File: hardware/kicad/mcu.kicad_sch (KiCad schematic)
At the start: 34 parts, among them J3 SWD, J4 UART, J5 Reset_Switch, SW2 PEC11R-4220F-S0024, U6 OLED, U7 STM32F072CBTx, U8 PCT2075GV, Y1 Crystal_8MHz

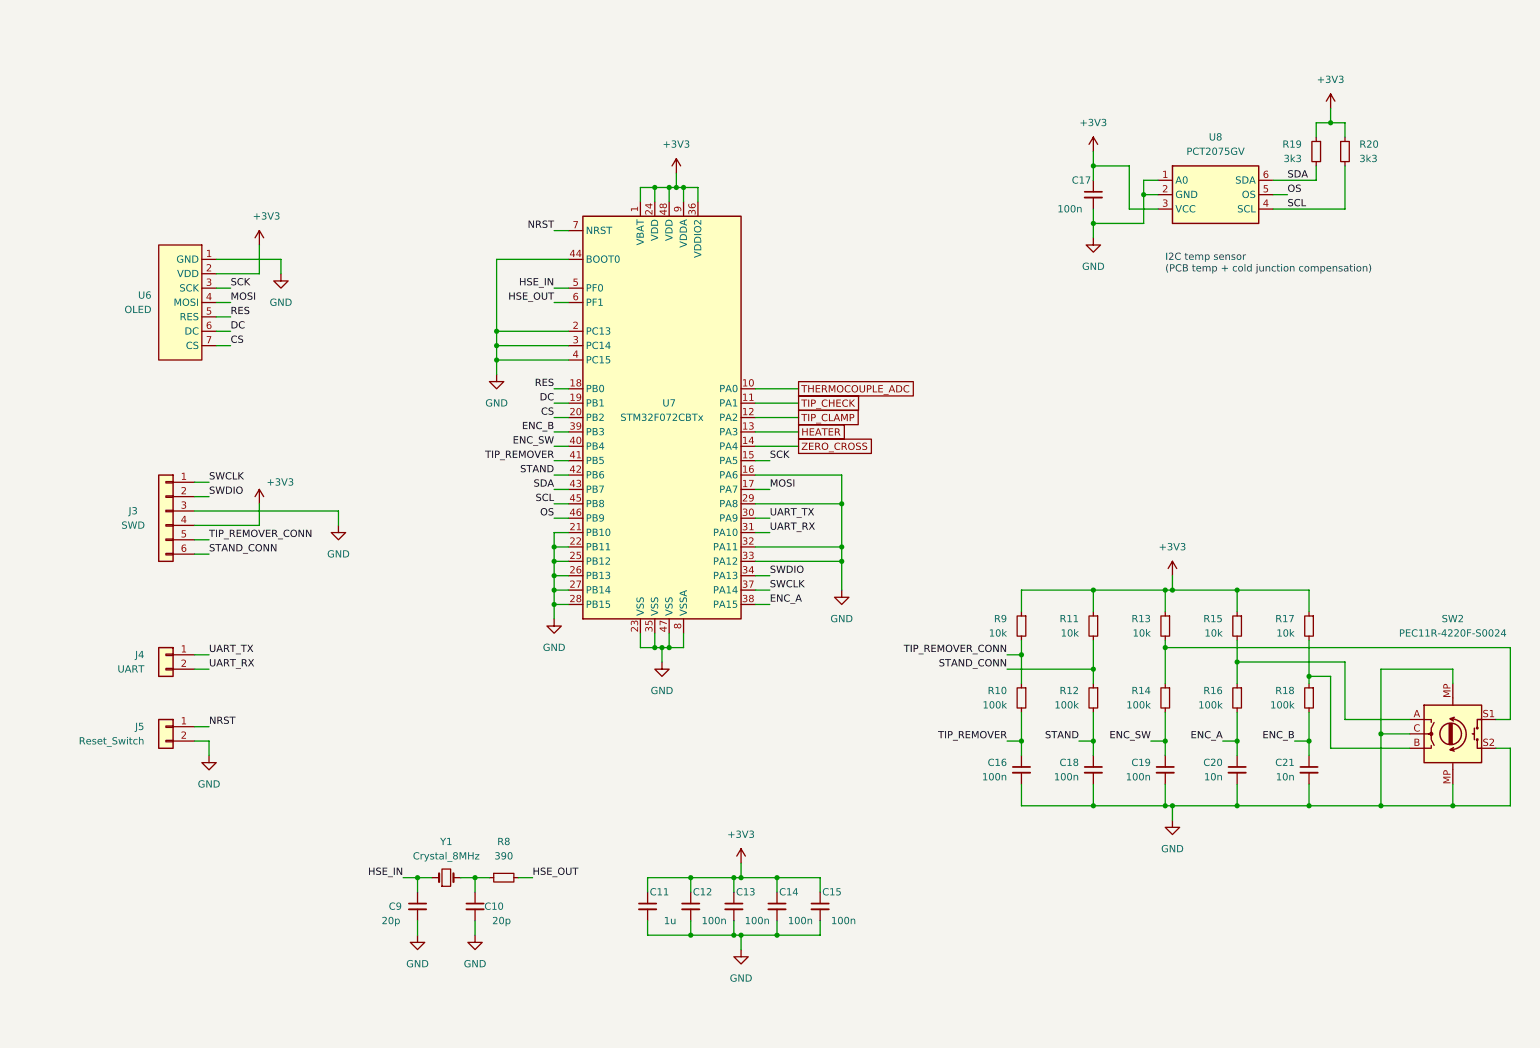
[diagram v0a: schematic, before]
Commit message: Schematic update.
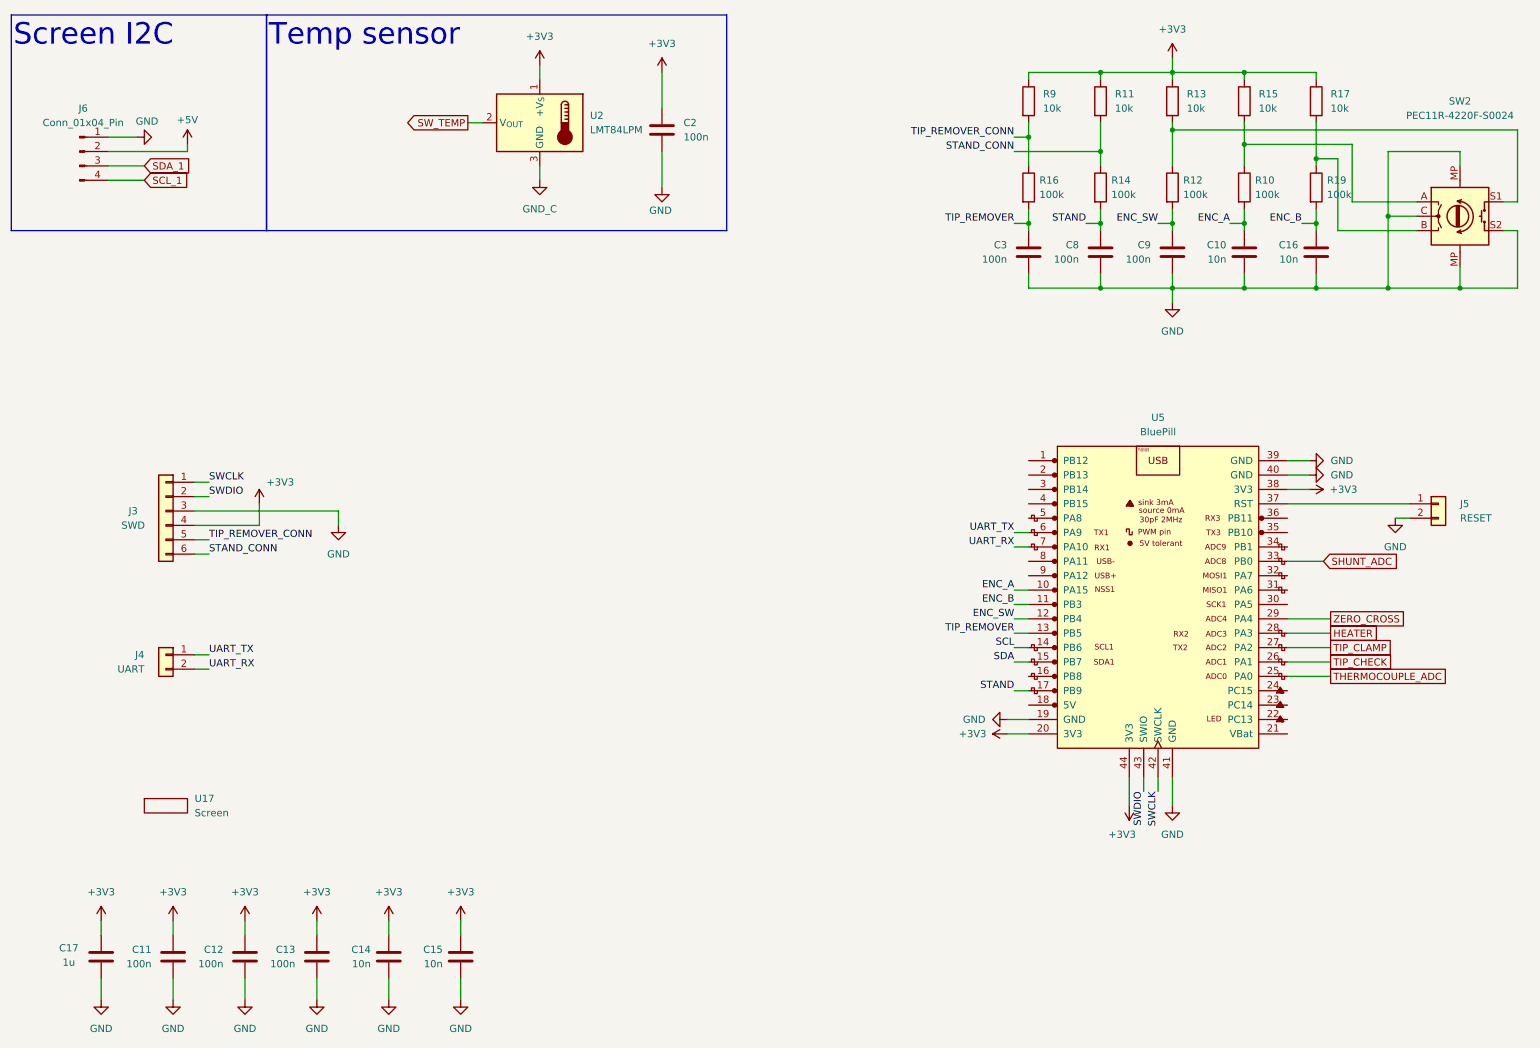
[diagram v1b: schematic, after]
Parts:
- removed C10, C9: 20p, Capacitor_SMD:C_0805_2012Metric, symbol Device:C_Small
- removed C11: 1u, Capacitor_SMD:C_1210_3225Metric, symbol Device:C_Small
- removed C12, C13, C14, C15, C16, C17, C18, C19: 100n, Capacitor_SMD:C_0805_2012Metric, symbol Device:C_Small
- removed C20, C21: 10n, Capacitor_SMD:C_0805_2012Metric, symbol Device:C_Small
- removed R10, R12, R14, R16, R18: 100k, Resistor_SMD:R_0805_2012Metric, symbol Device:R_Small
- removed R11, R13, R15, R17, R9: 10k, Resistor_SMD:R_0805_2012Metric, symbol Device:R_Small
- removed R19, R20: 3k3, Resistor_SMD:R_0805_2012Metric, symbol Device:R_Small
- removed R8: 390, Resistor_SMD:R_0805_2012Metric, symbol Device:R_Small
- removed U6: OLED, 0_Howie:OLED_SSD1306_SPI_1.54, symbol 0_Howie:OLED_SSD1306_SPI_1.54
- removed U7: STM32F072CBTx, Package_QFP:LQFP-48_7x7mm_P0.5mm, symbol MCU_ST_STM32F0:STM32F072CBTx
- removed U8: PCT2075GV, Package_SO:TSOP-6_1.65x3.05mm_P0.95mm, symbol 0_Howie:PCT2075GV
- removed Y1: Crystal_8MHz, Crystal:Crystal_SMD_HC49-SD, symbol 0_Howie:Crystal_8MHz
- added C10, C14, C15, C16: 10n, Capacitor_SMD:C_0603_1608Metric_Pad1.08x0.95mm_HandSolder, symbol Device:C
- added C11, C12, C13, C2, C3, C8, C9: 100n, Capacitor_SMD:C_0603_1608Metric_Pad1.08x0.95mm_HandSolder, symbol Device:C
- added C17: 1u, Capacitor_SMD:C_0603_1608Metric_Pad1.08x0.95mm_HandSolder, symbol Device:C
- added J6: Conn_01x04_Pin, Connector_PinHeader_2.54mm:PinHeader_1x04_P2.54mm_Vertical, symbol Connector:Conn_01x04_Pin
- added R10, R12, R14, R16, R19: 100k, Resistor_SMD:R_0603_1608Metric_Pad0.98x0.95mm_HandSolder, symbol Device:R
- added R11, R13, R15, R17, R9: 10k, Resistor_SMD:R_0603_1608Metric_Pad0.98x0.95mm_HandSolder, symbol Device:R
- added U17: Screen, opensolder:WC1602A, symbol PSG:20x4_screen
- added U2: LMT84LPM, Package_TO_SOT_THT:TO-92_Inline_W4.0mm_Horizontal_FlatSideDown, symbol Sensor_Temperature:LM35-LP
- added U5: BluePill, opensolder:BluePill, symbol opensolder:BluePill
- J5: value Reset_Switch -> RESET
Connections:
- net +3V3: now also C11.2, C12.2, C13.2, C14.2, C15.2, C17.1, C2.2, R11.1, R13.1, R15.1, R17.1, R9.1, U2.1 (+V_{S}), U5.20 (3V3), U5.38 (3V3), U5.44 (3V3)
- net ENC_A: now also C10.2, R10.2, U5.10 (PA15)
- net ENC_B: now also C16.2, R19.2, U5.11 (PB3)
- net ENC_SW: now also C9.2, R12.2, U5.12 (PB4)
- net GND: now also C10.1, C11.1, C12.1, C13.1, C14.1, C15.1, C16.1, C17.2, C2.1, C3.1, C8.1, C9.1, J6.1 (Pin_1), U5.19 (GND), U5.39 (GND), U5.40 (GND), U5.41 (GND)
- net HEATER: now also U5.28 (PA3)
- net SCL: now also U5.14 (PB6)
- net SDA: now also U5.15 (PB7)
- net STAND: now also C8.2, R14.2, U5.17 (PB9)
- net STAND_CONN: now also R11.2, R14.1
- net SWCLK: now also U5.42 (SWCLK)
- net SWDIO: now also U5.43 (SWIO)
- net THERMOCOUPLE_ADC: now also U5.25 (PA0)
- net TIP_CHECK: now also U5.26 (PA1)
- net TIP_CLAMP: now also U5.27 (PA2)
- net TIP_REMOVER: now also C3.2, R16.2, U5.13 (PB5)
- net TIP_REMOVER_CONN: now also R16.1, R9.2
- net UART_RX: now also U5.7 (PA10)
- net UART_TX: now also U5.6 (PA9)
- net ZERO_CROSS: now also U5.29 (PA4)
- net at SW2.B: now also R17.2, R19.1
- net at SW2.A: now also R10.1, R15.2
- net at SW2.S1: now also R12.1, R13.2
- net NRST: no longer names the net of J5.1 (Pin_1)
- net NRST: now also U5.37 (RST)
- new net +5V: J6.2 (Pin_2)
- new net GND_C: U2.3 (GND)
- new net SCL_1: J6.4 (Pin_4)
- new net SDA_1: J6.3 (Pin_3)
- new net SHUNT_ADC: U5.33 (PB0)
- new net SW_TEMP: U2.2 (V_{OUT})
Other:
- note added: "Screen I2C"
- note added: "Temp sensor"
- note removed: "I2C temp sensor (PCB temp + cold junction compensation)"
- moved on the sheet: SW2
